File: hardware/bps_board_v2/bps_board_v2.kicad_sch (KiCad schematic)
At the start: 62 parts, among them J1 USB_C_Receptacle_USB2.0_16P, J2 Conn_01x02, J4 Conn_01x02, Q1 DMG9926UDM, U2 DW01A, U3 MCP65R41, U4 TLV61048DBVR, U5 TLV61048DBVR, U8 4056 3PEAK, U9 OR Dual Diode

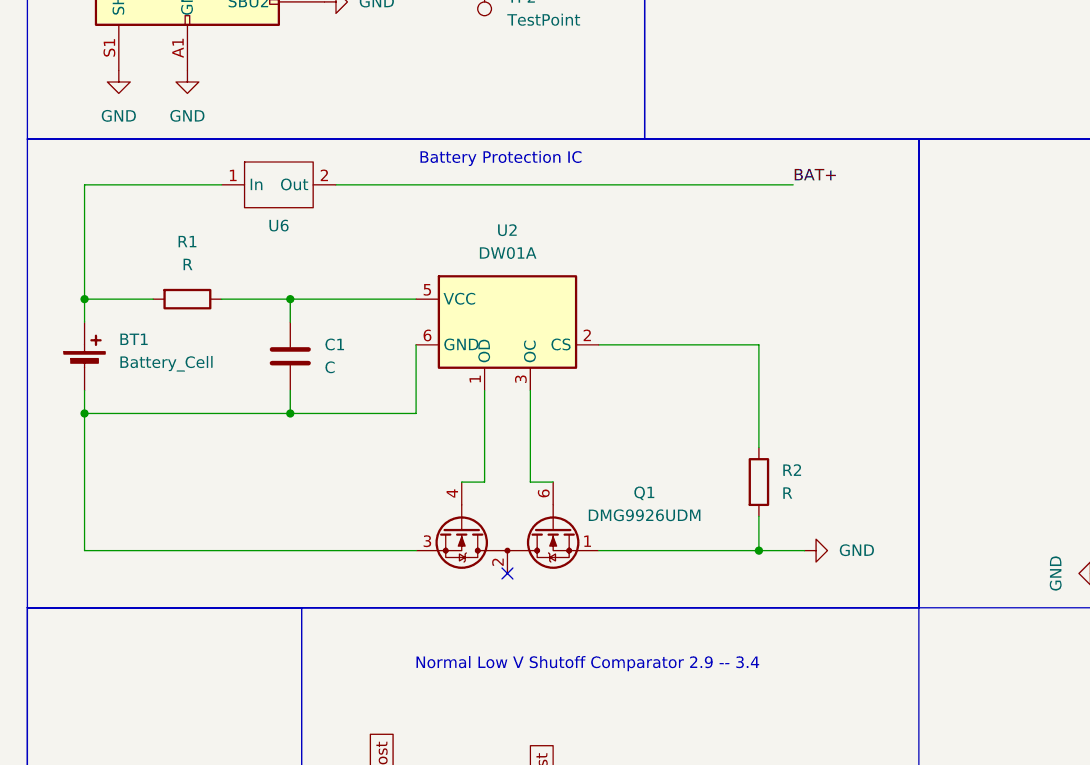
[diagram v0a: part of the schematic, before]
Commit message: Routing bps_board_v2
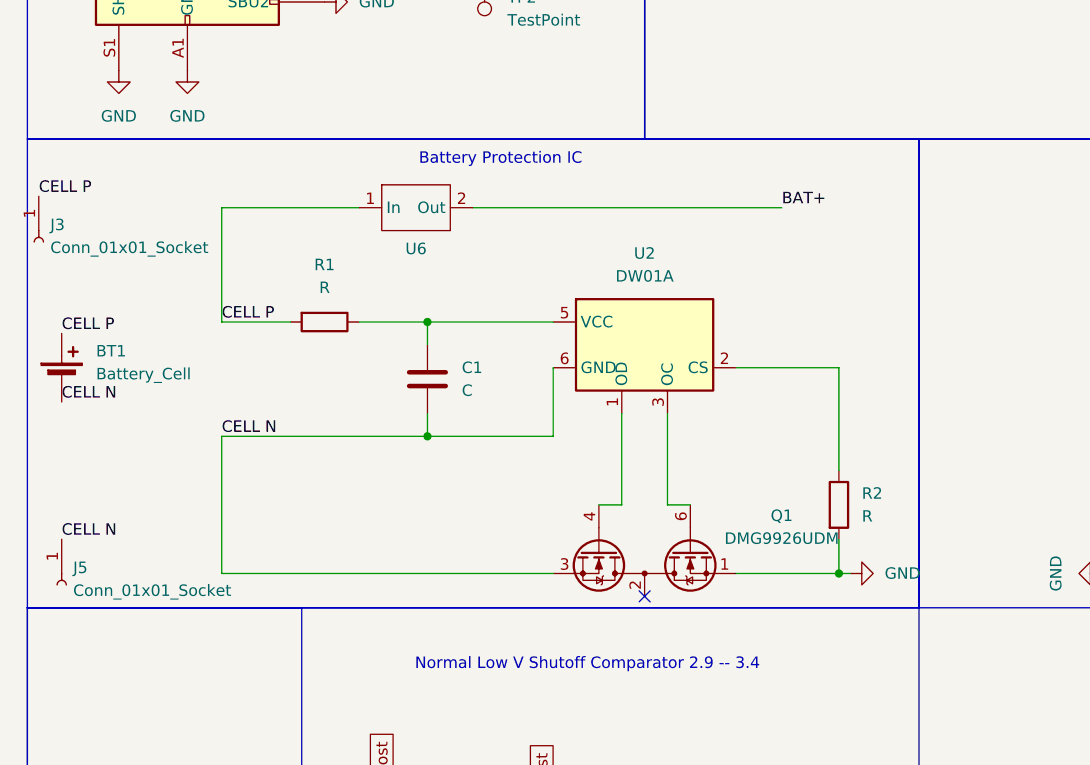
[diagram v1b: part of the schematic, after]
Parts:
- added J3, J5: Conn_01x01_Socket, GregFootprints:EmptyPad, symbol Connector:Conn_01x01_Socket
- H1, H2, H3, H4: footprint MountingHole:MountingHole_2.2mm_M2 -> MountingHole:MountingHole_3.2mm_M3
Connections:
- net CELL P: now reaches BT1.1 (+), R1.2, U6.1 (In)
- net CELL P: now also J3.1 (Pin_1)
- net CELL N: now reaches BT1.2 (-), C1.2, Q1.3 (S2), U2.6 (GND)
- net CELL N: now also J5.1 (Pin_1)
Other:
- moved on the sheet: BT1, C1, Q1, R1, R2, U2, U6
